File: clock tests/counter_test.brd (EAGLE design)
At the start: 100 x 75 mm, 29 parts, among them IC3 74LS08N, IC4 74LS11N, IC5 74S260D, IC6 74LS112D

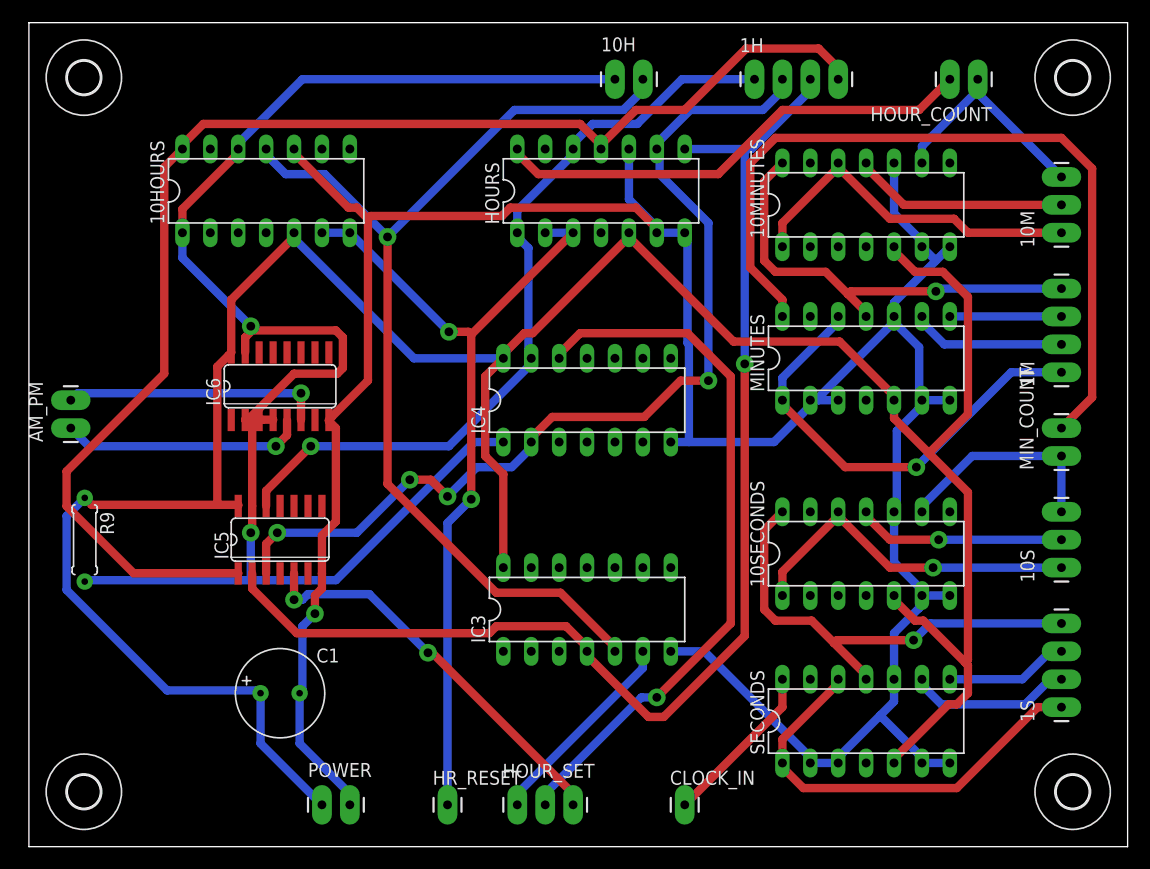
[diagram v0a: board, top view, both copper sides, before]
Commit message: clock pulse test new
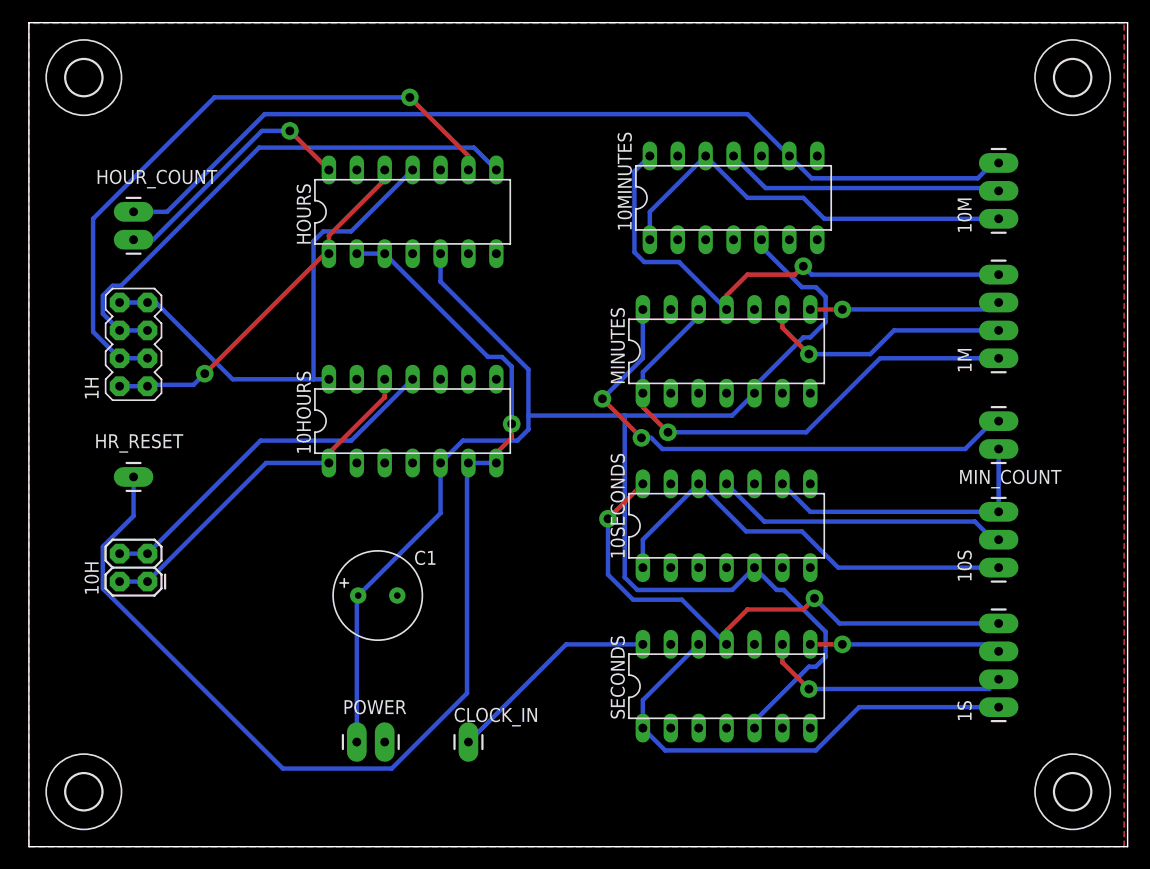
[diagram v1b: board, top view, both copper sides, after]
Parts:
- removed AM_PM: (no value), iStivi - Header-Connector:1X02_LONGPADS
- removed HOUR_SET: (no value), iStivi - Header-Connector:1X03_LONGPADS
- removed IC3: 74LS08N, iStivi - ICs:DIL14
- removed IC4: 74LS11N, iStivi - ICs:DIL14
- removed IC5: 74S260D, iStivi - ICs:SO14
- removed IC6: 74LS112D, iStivi - ICs:SO16
- removed R9: 10K, iStivi - RCLD:0207/7
- removed U$2, U$3, U$4: (no value), iStivi - Board-Holes:3,0
- 10H: device iStivi - Header-Connector:1X02_LONGPADS -> iStivi - Header-Connector:2X2
- 1H: device iStivi - Header-Connector:1X04_LONGPADS -> iStivi - Header-Connector:2X4
- CLOCK_IN: value M01PTH_LONGPAD -> (none)
- U$1: device iStivi - Board-Holes:3,0 -> iStivi - Board-templates:BOARD-75X100
- moved HOUR_COUNT 77.8 mm to (9.53, 57.8), turned to 270 degrees
- moved U$1 70.2 mm to (0.00, 0.00)
- moved 10H 62.4 mm to (9.53, 25.4), turned to 90 degrees
- moved 1H 61.5 mm to (9.53, 45.7), turned to 90 degrees
- moved HR_RESET 41.3 mm to (9.53, 33.7), turned to 90 degrees
- moved 10HOURS 24.8 mm to (34.9, 38.7)
- moved CLOCK_IN 20.5 mm to (40.0, 9.53)
- moved HOURS 17.3 mm to (34.9, 57.8)
- moved SECONDS 13.1 mm to (63.5, 14.6)
- moved 10SECONDS 13.0 mm to (63.5, 29.2)
- moved MINUTES 12.7 mm to (63.5, 45.1)
- moved C1 12.6 mm to (31.8, 22.9)
- moved 10MINUTES 12.1 mm to (64.1, 59.1)
- moved POWER 6.54 mm to (29.8, 9.53)
- moved 1M 5.85 mm to (88.3, 44.5)
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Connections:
- removed net 12_HR: HOUR_SET.2, IC4.12
- removed net 24_HR: HOUR_SET.1, IC3.6
- removed net AM: AM_PM.1, IC6.5
- removed net N$2: HOUR_SET.3, IC5.5
- removed net PM: AM_PM.2, IC6.6
- net 10H_A: now also 10H.2; no longer IC4.1, IC5.13, IC6.15, IC6.2, IC6.3, IC6.4, R9.2
- net 10H_B: now also 10H.3, 10H.4; no longer 10H.2, IC3.5
- net 1H_A: now also 1H.2; no longer IC4.13, IC5.12
- net 1H_B: now also 1H.3, 1H.4; no longer 1H.2, IC4.2, IC5.3
- net 1H_C: now also 1H.5, 1H.6; no longer 1H.3, IC3.4, IC5.2
- net 1H_D: now also 1H.7, 1H.8; no longer 1H.4, IC5.1
- net GND: no longer IC3.7, IC4.7, IC5.7, IC6.8
- net VCC: no longer IC3.14, IC4.14, IC5.14, IC6.16, R9.1
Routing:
- net GND: track 253.9 -> 0.00 mm, vias 1 -> 0
- net 10H_A: track 143.1 -> 33.2 mm, vias 2 -> 0
- net VCC: track 250.1 -> 147.3 mm
- net 1H_D: track 122.9 -> 46.2 mm
- net 1H_C: track 114.1 -> 48.6 mm, vias 1 -> 0
- net 12_HR: track 65.2 -> 0.00 mm, vias 1 -> 0
- net 10M_C: track 21.7 -> 85.4 mm
- net 10H_B: track 94.2 -> 33.2 mm, vias 1 -> 0
- net 1H_A: track 72.2 -> 34.0 mm
- net N$2: track 36.5 -> 0.00 mm, vias 2 -> 0
- net 1H_B: track 88.9 -> 58.5 mm, vias 4 -> 1
- net HR_RESET: track 76.8 -> 105.3 mm, vias 2 -> 1
- net N$1: track 73.2 -> 48.7 mm, vias 0 -> 2
- net PM: track 23.7 -> 0.00 mm, vias 1 -> 0
- net AM: track 22.2 -> 0.00 mm, vias 1 -> 0
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- added copper zone on layer 1, net GND
- added copper zone on layer 16, net GND
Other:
- board text removed: "+5V"
- board text removed: "10HR"
- board text removed: "10MIN"
- board text removed: "10SEC"
- board text removed: ">H"
- board text removed: ">M"
- board text removed: "A"
- board text removed: "AM/PM"
- board text removed: "B"
- board text removed: "C"
- board text removed: "CLK"
- board text removed: "D"
- board text removed: "GND"
- board text removed: "H>"
- board text removed: "HR"
- board text removed: "HR_RESET"
- board text removed: "M>"
- board text removed: "MIN"
- board text removed: "SEC"
